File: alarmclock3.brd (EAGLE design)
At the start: 81 x 80 mm, 28 parts, among them X1 MKDSN1,5/2-5,08, X2 MKDSN1,5/2-5,08

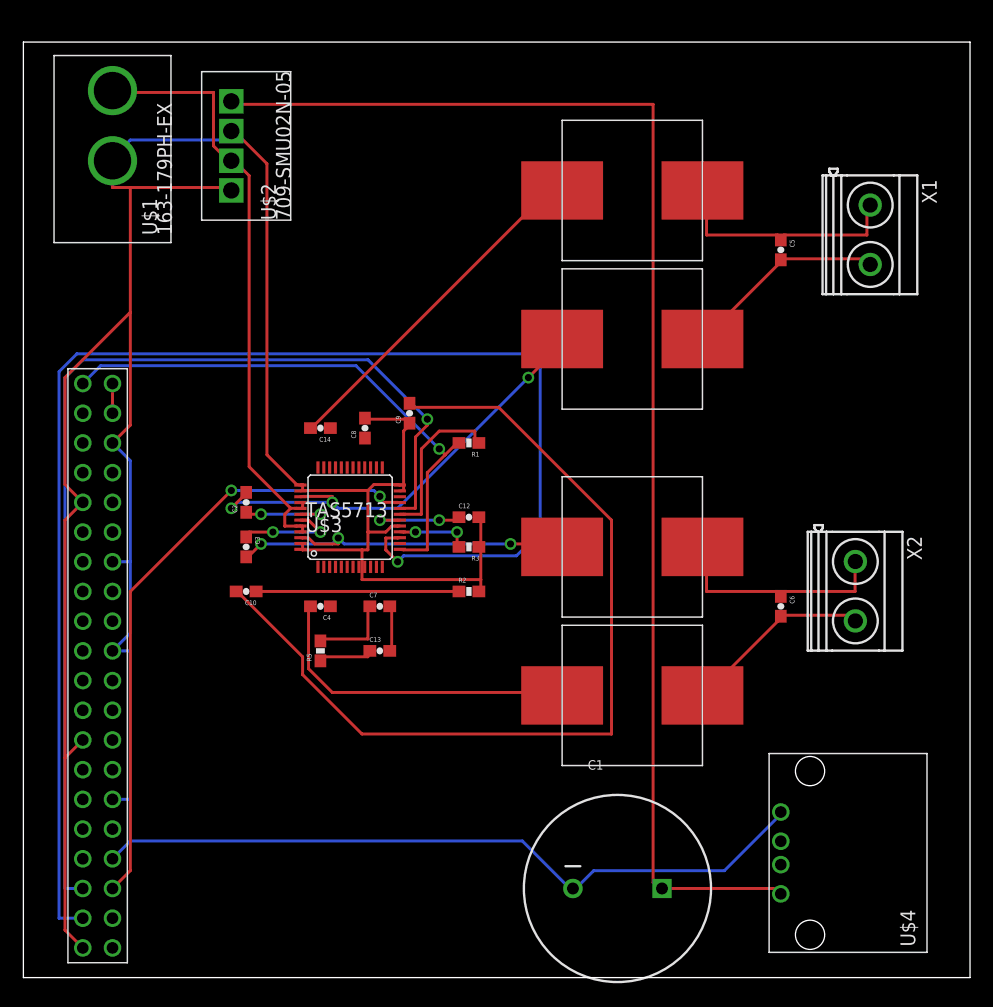
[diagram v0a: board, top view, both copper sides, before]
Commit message: route 100%
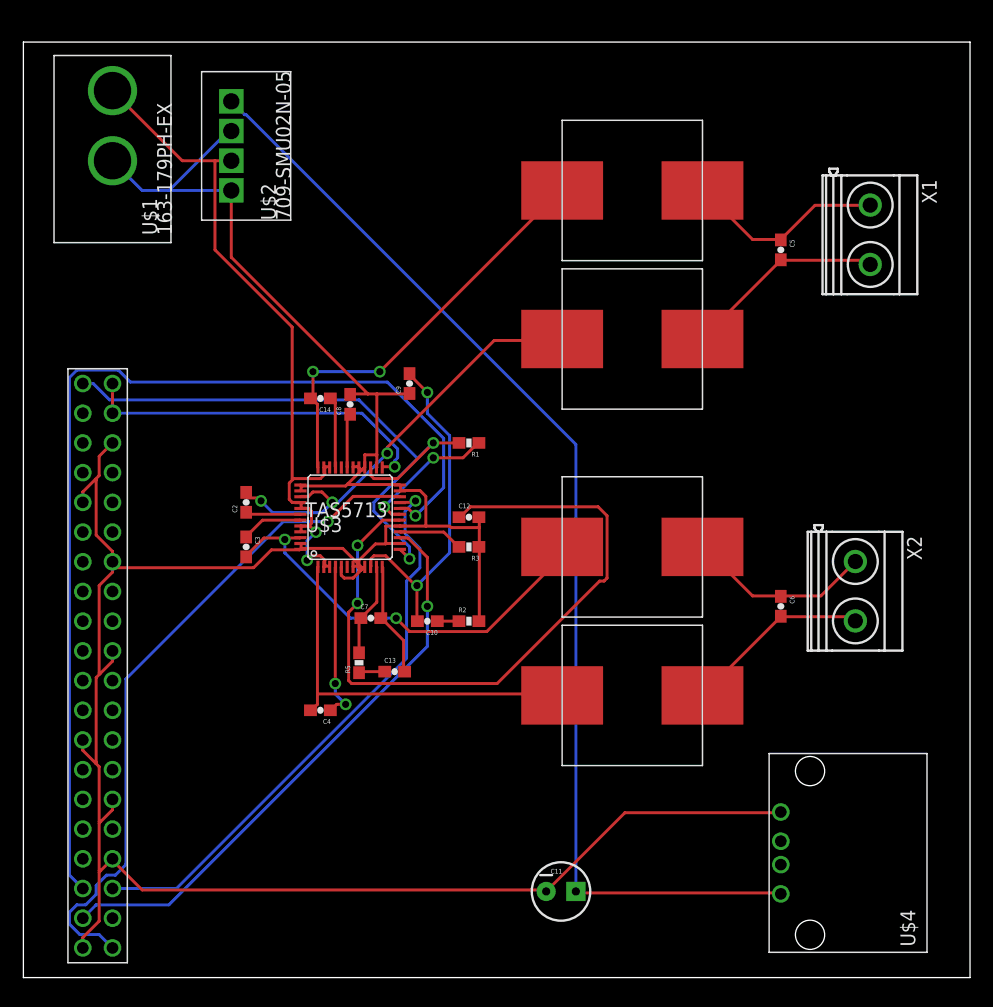
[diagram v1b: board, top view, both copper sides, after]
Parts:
- removed C1: (no value), SparkFun-Passives:CPOL-RADIAL-1000UF-63V
- added C11: 330uF/25V, SparkFun-Passives:CPOL-RADIAL-10UF-25V
- moved C10 15.7 mm to (34.5, 30.5)
- moved C4 8.89 mm to (25.4, 22.9)
- moved R5 3.45 mm to (28.7, 26.9)
- moved R2 2.54 mm to (38.1, 30.5)
- moved C14 2.54 mm to (25.4, 49.5)
- moved C9 2.54 mm to (33.0, 50.8)
- moved C8 2.40 mm to (27.9, 49.0)
- moved C13 2.18 mm to (31.8, 26.2)
- moved C7 1.27 mm to (29.7, 30.7)
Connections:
- net GND: now also C11.2; no longer C1.2
- net N$3: now also C11.1; no longer C1.1
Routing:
- net N$2: track 122.7 -> 49.8 mm
- net N$1: track 0.00 -> 58.3 mm, vias 0 -> 1
- net GND: track 297.0 -> 241.2 mm
- net N$27: track 8.62 -> 61.0 mm
- net N$23: track 77.9 -> 29.6 mm, vias 0 -> 2
- net N$8: track 2.54 -> 30.9 mm, vias 0 -> 1
- net N$3: track 114.3 -> 97.5 mm
- net N$25: track 17.4 -> 1.86 mm
- net N$12: track 0.00 -> 13.6 mm, vias 0 -> 2
- net N$6: track 47.5 -> 55.3 mm, vias 1 -> 2
- net VCC: track 53.8 -> 60.4 mm, vias 0 -> 2
- net N$10: track 29.9 -> 36.4 mm, vias 0 -> 2
- net N$11: track 0.00 -> 6.11 mm
- net N$22: track 4.03 -> 9.95 mm
- net N$13: track 28.0 -> 33.5 mm
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
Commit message: !00% routable
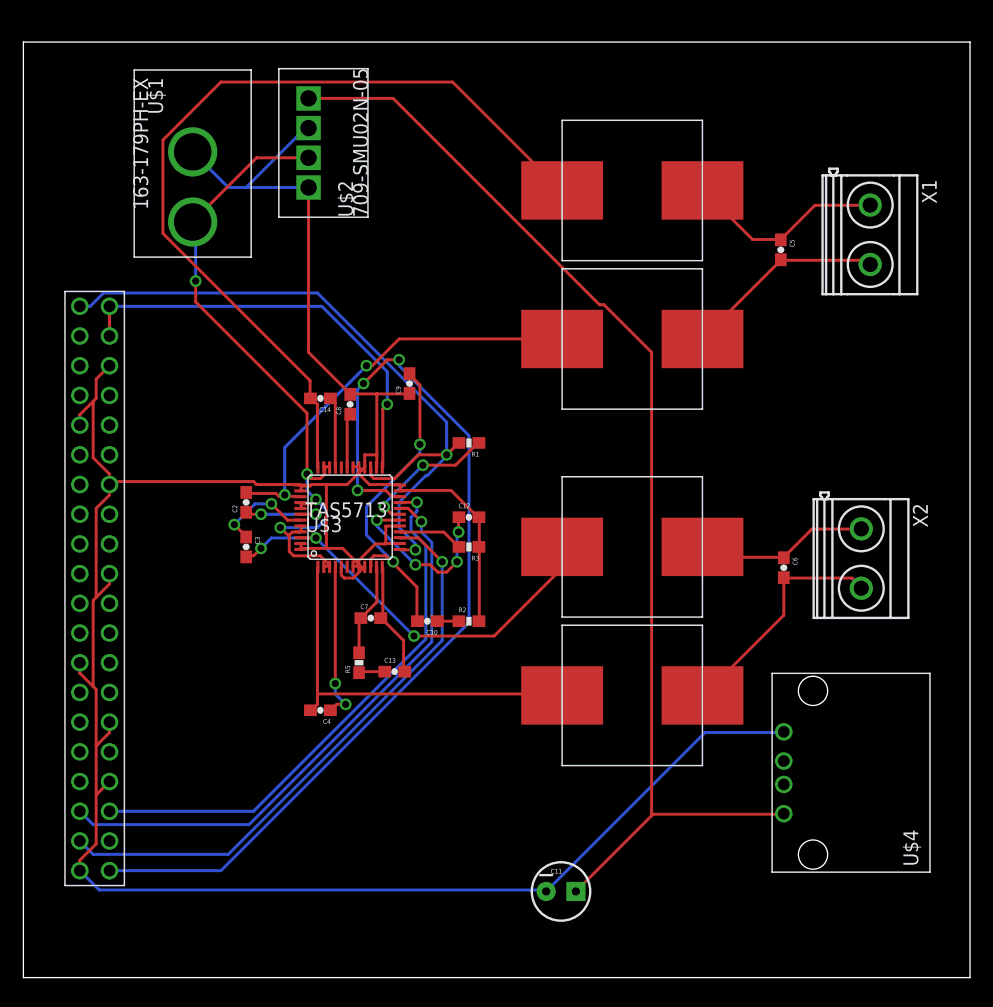
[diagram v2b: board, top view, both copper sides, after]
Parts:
- moved U$1 6.90 mm to (14.5, 70.6), turned to 270 degrees
- moved U$4 6.86 mm to (65.0, 17.0)
- moved U$2 6.61 mm to (24.4, 72.6)
- moved U$5 6.61 mm to (6.10, 47.2)
- moved C6 3.31 mm to (65.0, 35.1)
- moved X2 2.84 mm to (71.6, 35.8)
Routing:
- net N$27: track 61.0 -> 15.2 mm, vias 2 -> 4
- net N$4: track 88.1 -> 50.0 mm
- net N$10: track 36.4 -> 73.6 mm, vias 2 -> 0
- net N$1: track 58.3 -> 81.5 mm, vias 1 -> 3
- net N$8: track 30.9 -> 37.0 mm
- net N$6: track 55.3 -> 60.6 mm
- net N$18: track 16.2 -> 20.0 mm
- net N$15: track 5.26 -> 8.45 mm, vias 0 -> 2
- net N$17: track 4.73 -> 7.39 mm, vias 0 -> 2
- net GND: track 241.2 -> 243.8 mm
- net N$5: track 49.5 -> 47.0 mm
- net N$23: track 29.6 -> 28.2 mm
- net N$9: track 16.1 -> 15.0 mm
- net N$16: track 37.7 -> 36.6 mm, vias 3 -> 2
- net N$3: track 97.5 -> 98.5 mm
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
